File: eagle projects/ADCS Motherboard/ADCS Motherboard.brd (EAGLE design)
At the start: 91 x 91 mm, 141 parts, among them J1 HDR_10_EZFET_DEBUGGER, J11 CNC_3221-10-0300-00, J5 CNC_3221-10-0300-00, J7 TE-1734829-3, Q1 BSR802NL6327HTSA1, U1 MSP430F5529IPN, U10 TSV991AILT, U2 TSV991AILT, U3 ADS7841E_2K5, U4 TSV991AILT, U5 DMC4050SSDQ-13, U7 HMC1053, U9 BMX160, Y1 32.768kHz, Y2 CSTCR4M00G15L99, Y3 32.768kHz

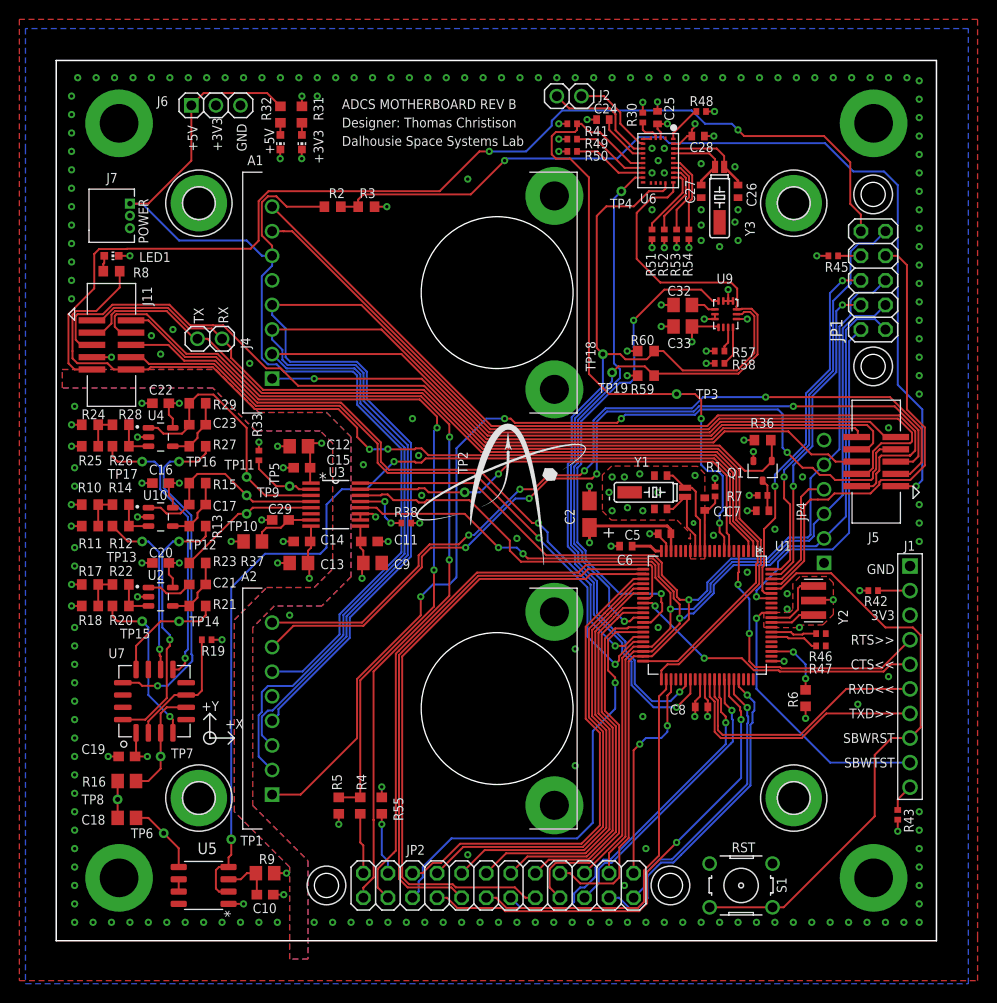
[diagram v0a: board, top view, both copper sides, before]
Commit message: I thinks its done
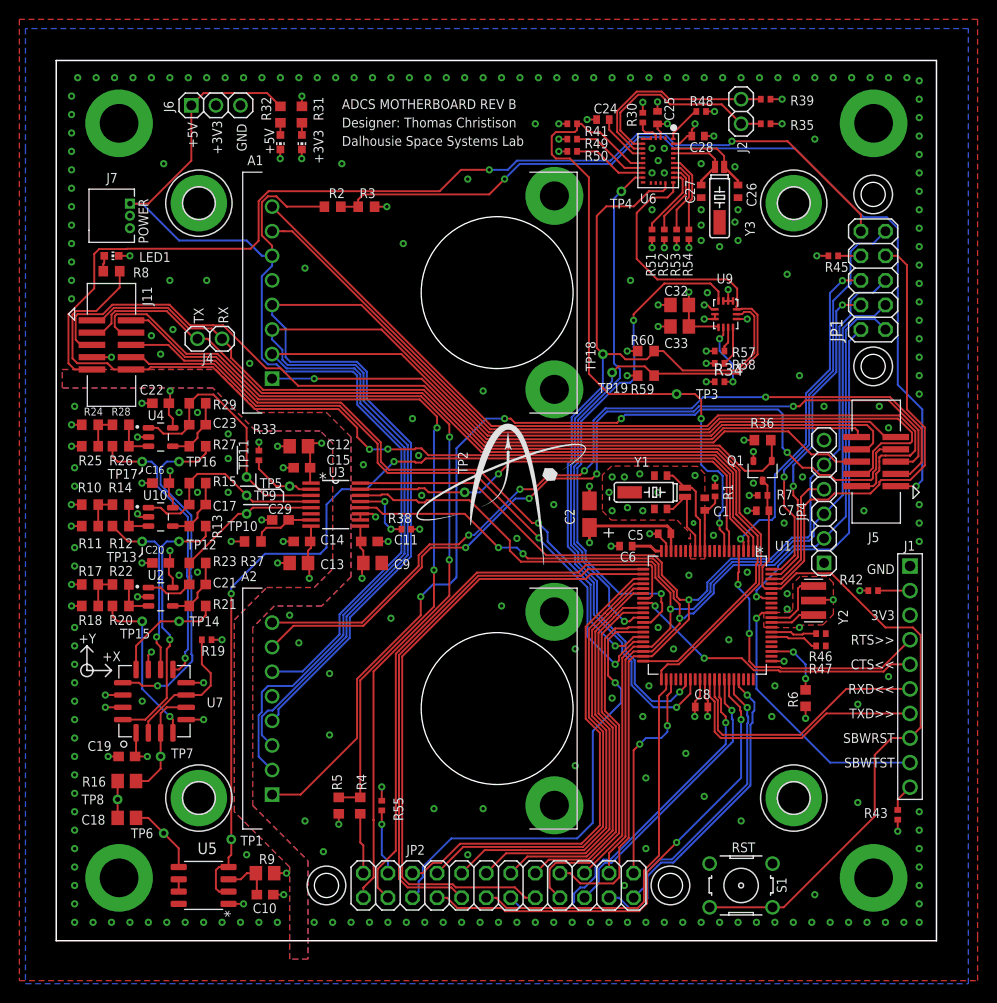
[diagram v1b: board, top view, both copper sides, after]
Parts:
- added R34, R35, R39: 5.1M, rcl:R0402
- R37: device rcl:R0805 -> rcl:R0603
- R55: device rcl:R0603 -> rcl:R0402
- U6: value (none) -> BNO055
- moved J2 17.9 mm to (70.8, 85.7), turned to 90 degrees
- moved R38 0.63 mm to (36.2, 42.5)
- moved C32 0.32 mm to (64.5, 65.7)
- moved C33 0.32 mm to (64.5, 63.5)
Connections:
- removed net N$2: C32.1, U9.5
- removed net N$41: U1.44
- removed net TB0.3: U1.58
- removed net TB0.4: U1.59
- net !CS!_SUN_Z-: now also U1.3; no longer U1.75
- net +3V3: now also C32.1, U9.5
- net BMX160_INT2: now also R34.2
- net GND: now also R34.1, R35.1, R39.1
- net N$16: now also R35.2
- net N$17: now also R39.2
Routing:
- net GND: track 71.8 -> 84.7 mm, vias 253 -> 311
- net N$16: track 9.09 -> 21.3 mm
- net N$17: track 12.2 -> 21.6 mm
- net RST/SBWTDIO: track 64.9 -> 74.1 mm
- net BMX160_INT2: track 0.00 -> 7.23 mm, vias 0 -> 2
- net Z-_SUN_3V_PRESENT: track 111.9 -> 107.5 mm
- net CAM_5V_PRESENT: track 99.4 -> 95.0 mm
- net +3V3: track 74.2 -> 78.6 mm, vias 25 -> 26
- net !CS!_SUN_Z-: track 38.5 -> 35.1 mm
- net N$2: track 2.57 -> 0.00 mm
- net B_MEAS_X: track 19.8 -> 22.0 mm
- net N$36: track 12.8 -> 14.3 mm
- net BMX160_INT1: track 52.4 -> 53.8 mm
- net CAMERA-2_CS: track 102.9 -> 101.6 mm
- net RW_Y_LOCK: track 67.2 -> 66.3 mm
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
